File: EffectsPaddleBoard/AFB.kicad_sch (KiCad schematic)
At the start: 25 parts, among them J5 AudioJack2, J6 AudioJack2, U5 MCP6401T-xLT, U6 MCP6401T-xLT, U7 MCP6401T-xLT

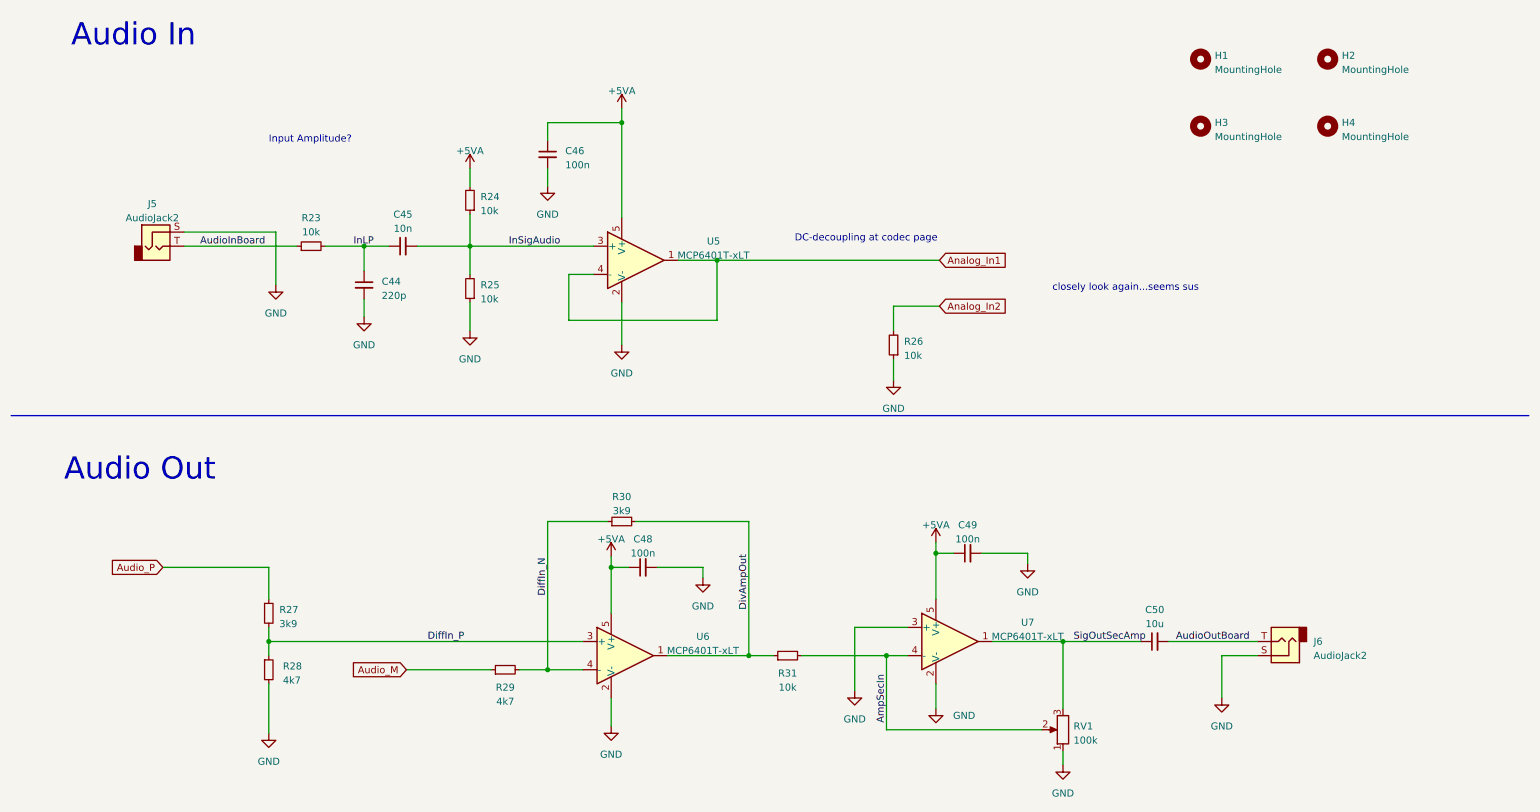
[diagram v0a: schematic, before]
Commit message: Reworked schematic completely, design will be next, if someone knows, where my branches went, tell me
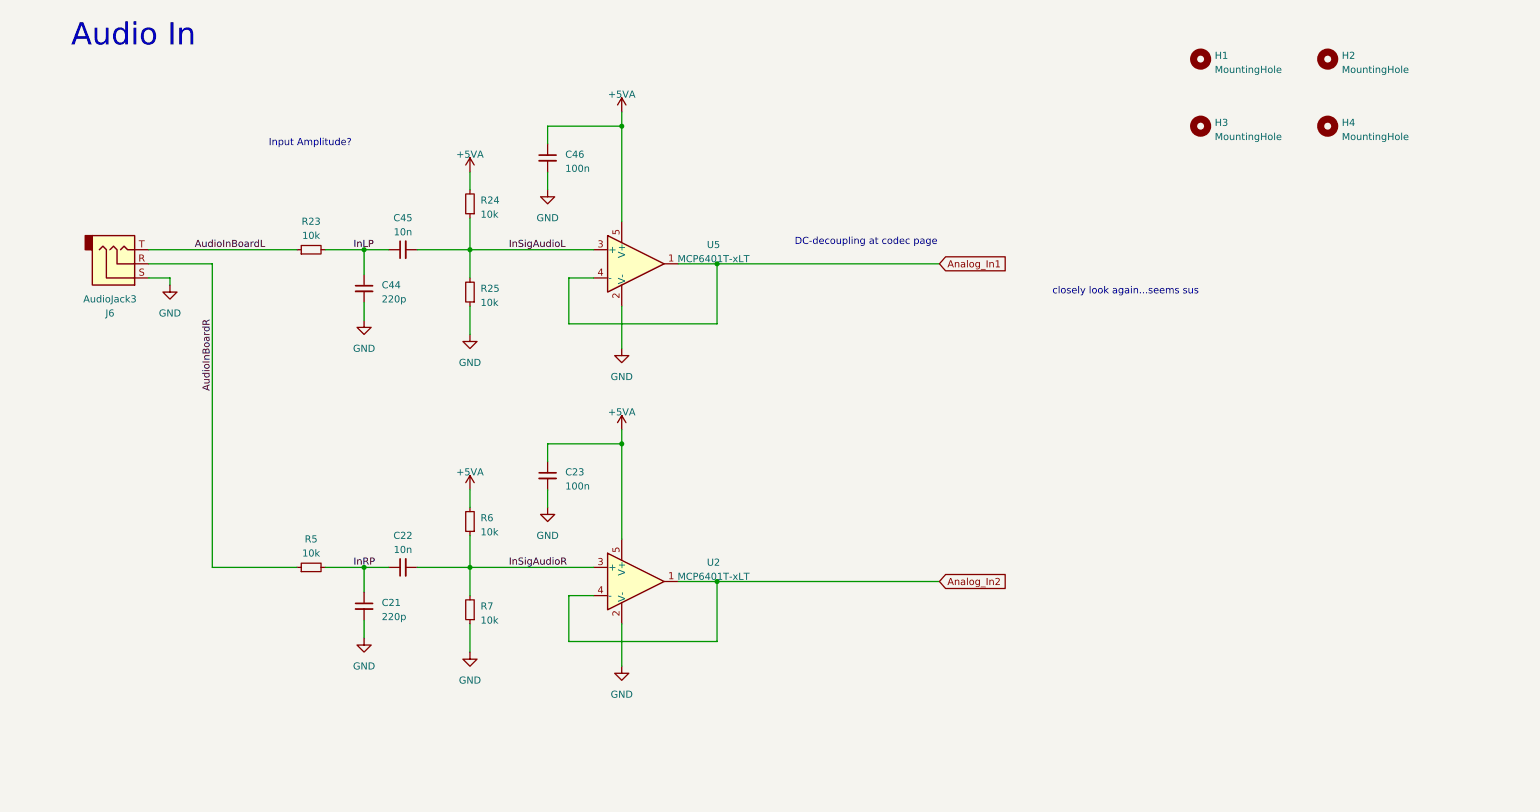
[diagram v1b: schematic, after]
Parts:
- removed C48, C49: 100n, Capacitor_SMD:C_0402_1005Metric, symbol Device:C_Small
- removed C50: 10u, Capacitor_SMD:C_1206_3216Metric, symbol Device:C_Small
- removed J5, J6: AudioJack2, Connector_Audio:Jack_6.35mm_Neutrik_NJ2FD-V_Vertical, symbol Connector_Audio:AudioJack2
- removed R26, R31: 10k, Resistor_SMD:R_0402_1005Metric, symbol Device:R_Small
- removed R27, R30: 3k9, Resistor_SMD:R_0402_1005Metric, symbol Device:R_Small
- removed R28, R29: 4k7, Resistor_SMD:R_0402_1005Metric, symbol Device:R_Small
- removed RV1: 100k, Potentiometer_THT:Potentiometer_Bourns_3005_Horizontal, symbol Device:R_Potentiometer
- removed U6, U7: MCP6401T-xLT, Package_TO_SOT_SMD:SOT-353_SC-70-5, symbol Amplifier_Operational:MCP6401T-xLT
- added C21: 220p, Capacitor_SMD:C_0402_1005Metric, symbol Device:C_Small
- added C22: 10n, Capacitor_SMD:C_0402_1005Metric, symbol Device:C_Small
- added C23: 100n, Capacitor_SMD:C_0402_1005Metric, symbol Device:C_Small
- added J6: AudioJack3, Connector_Audio:Jack_3.5mm_CUI_SJ1-3533NG_Horizontal_CircularHoles, symbol Connector_Audio:AudioJack3
- added R5, R6, R7: 10k, Resistor_SMD:R_0402_1005Metric, symbol Device:R_Small
- added U2: MCP6401T-xLT, Package_TO_SOT_SMD:SOT-353_SC-70-5, symbol Amplifier_Operational:MCP6401T-xLT
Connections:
- net +5VA: now also C23.1, R6.2, U2.5 (V+)
- net Analog_In2: now also U2.1, U2.4 (-)
- net GND: now also C21.2, C23.2, J6.S, R7.1, U2.2 (V-)
- net AudioInBoard renamed AudioInBoardL
- net AudioInBoardL: now also J6.T
- net InSigAudio renamed InSigAudioL
- new net AudioInBoardR: J6.R, R5.1
- new net InRP: C21.1, C22.1, R5.2
- new net InSigAudioR: C22.2, R6.1, R7.2, U2.3 (+)
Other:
- note removed: "Audio Out"
- moved on the sheet: C44, C45, C46, R23, R24, R25, U5
